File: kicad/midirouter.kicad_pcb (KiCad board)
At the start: 2 copper layers, 152.9 x 47.2 mm, 33 parts, among them J1 Conn_02x05_Odd_Even, J2 Conn_01x08, J3 Conn_01x08, J4 Conn_01x08, J5 Conn_01x08, J6 Conn_01x08, J7 Conn_01x08, J8 Conn_01x08, J9 Conn_01x08, Q1 PN2222A, Q2 PN2222A, Q3 PN2222A, Q4 PN2222A, U5 74LS595, U6 74LS595, U7 CMOD-A7, U8 L7805

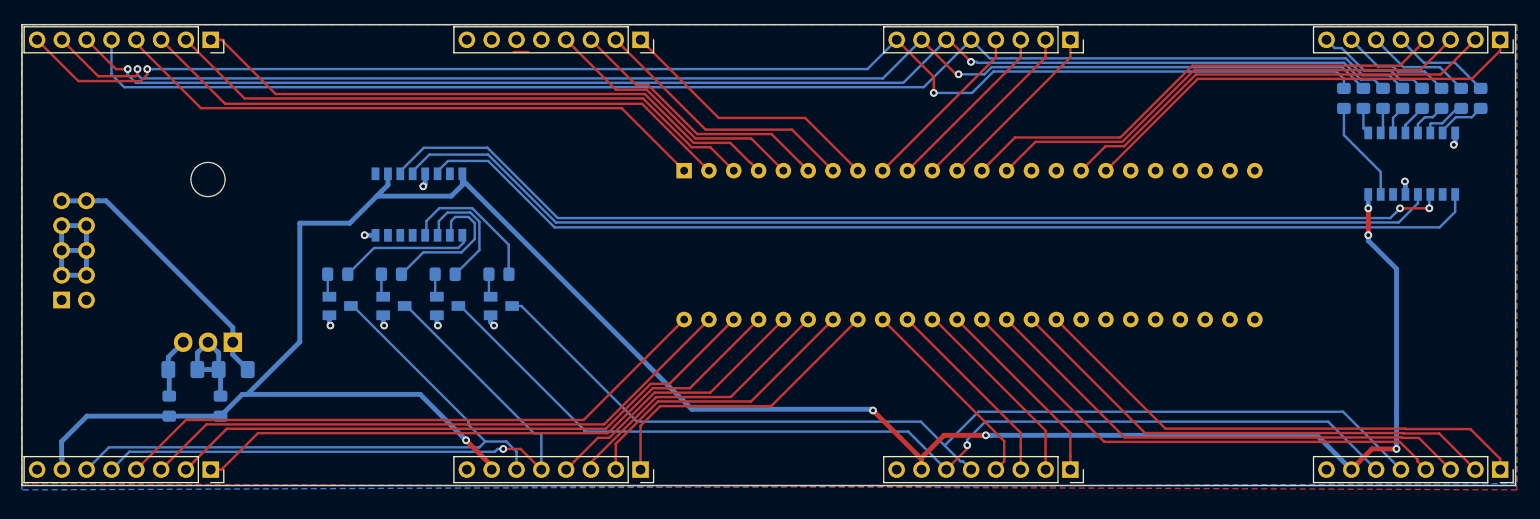
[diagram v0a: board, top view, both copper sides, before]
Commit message: More work on pcbs and frontpanel.
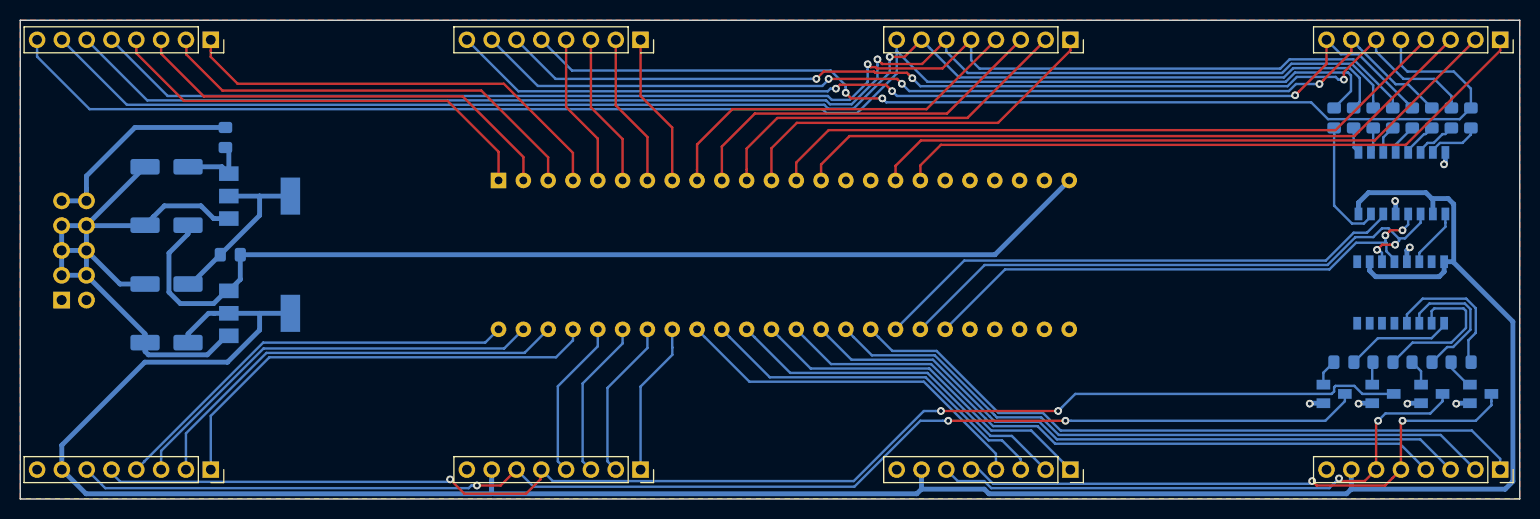
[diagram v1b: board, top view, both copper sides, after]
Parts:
- removed R77: 2K2, Resistor_SMD:R_0805_2012Metric_Pad1.15x1.40mm_HandSolder
- removed R78: 3K3, Resistor_SMD:R_0805_2012Metric_Pad1.15x1.40mm_HandSolder
- removed U8: L7805, Package_TO_SOT_THT:TO-220-3_Horizontal_TabDown
- added C1: C, Capacitor_SMD:CP_Elec_5x3.9, B.Cu at (41.5, 65.0)
- added C2: C, Capacitor_SMD:CP_Elec_5x3.9, B.Cu at (41.5, 77.0)
- added D1: D, Diode_SMD:D_0805_2012Metric_Pad1.15x1.40mm_HandSolder, B.Cu at (48.0, 68.0)
- added D2: D, Diode_SMD:D_0805_2012Metric_Pad1.15x1.40mm_HandSolder, B.Cu at (47.5, 56.0)
- added U1: LD1117S50TR_SOT223, Package_TO_SOT_SMD:SOT-223-3_TabPin2, B.Cu at (51.0, 62.0)
- added U2: LD1117S33TR_SOT223, Package_TO_SOT_SMD:SOT-223-3_TabPin2, B.Cu at (51.0, 74.0)
- C17, C18: footprint Capacitor_SMD:C_1206_3216Metric_Pad1.42x1.75mm_HandSolder -> Capacitor_SMD:CP_Elec_5x3.9
- moved R25 103.4 mm to (162.0, 79.0)
- moved Q4 102.1 mm to (161.0, 82.2)
- moved R26 101.9 mm to (166.0, 79.0)
- moved Q3 101.6 mm to (166.0, 82.2)
- moved Q2 101.2 mm to (171.0, 82.2)
- moved U6 100.9 mm to (167.8, 71.9)
- moved Q1 100.7 mm to (176.0, 82.2)
- moved R27 100.4 mm to (170.0, 79.0)
- moved R28 98.9 mm to (174.0, 79.0)
- moved C17 21.8 mm to (41.5, 59.0)
- moved U7 19.0 mm to (78.0, 67.0)
- moved C18 8.91 mm to (41.5, 71.0), turned to 180 degrees
- moved R17 2.24 mm to (161.0, 54.0)
- moved R18 2.24 mm to (163.0, 54.0)
- moved R19 2.24 mm to (165.0, 54.0)
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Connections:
- C17 pad 1: +12V -> Net-(C17-Pad1)
- C18 pad 1: +5V -> Net-(C18-Pad1)
- U7 pad 24: +5V -> CA7_VCC
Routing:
- net CA7_VCC: track 0.00 -> 108.0 mm
- net Net-(U5-Pad9): track 110.1 -> 5.99 mm
- net LED8: track 10.2 -> 112.2 mm, vias 0 -> 2
- net LED5: track 11.8 -> 106.4 mm, vias 0 -> 3
- net LED7: track 10.9 -> 105.2 mm, vias 0 -> 3
- net LED6: track 11.3 -> 104.9 mm, vias 0 -> 3
- net LEDK2: track 68.9 -> 139.4 mm, vias 1 -> 3
- net LEDK1: track 67.1 -> 135.5 mm, vias 0 -> 3
- net Net-(U5-Pad14): track 0.00 -> 55.0 mm
- net Net-(U5-Pad12): track 108.5 -> 55.8 mm, vias 0 -> 2
- net Net-(U5-Pad11): track 111.5 -> 61.9 mm
- net LEDK3: track 105.6 -> 59.1 mm, vias 1 -> 2
- net LEDK4: track 104.5 -> 61.6 mm, vias 0 -> 2
- net GND: track 39.0 -> 79.4 mm, vias 8 -> 7
- net MIDI_IN_12: track 18.2 -> 39.1 mm
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- removed copper zone on B.Cu, net GND
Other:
- board size 152.9 x 47.2 mm -> 153.5 x 49 mm
